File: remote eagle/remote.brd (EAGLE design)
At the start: 36.8 x 36.8 mm, 13 parts, among them U1 BLE112-A

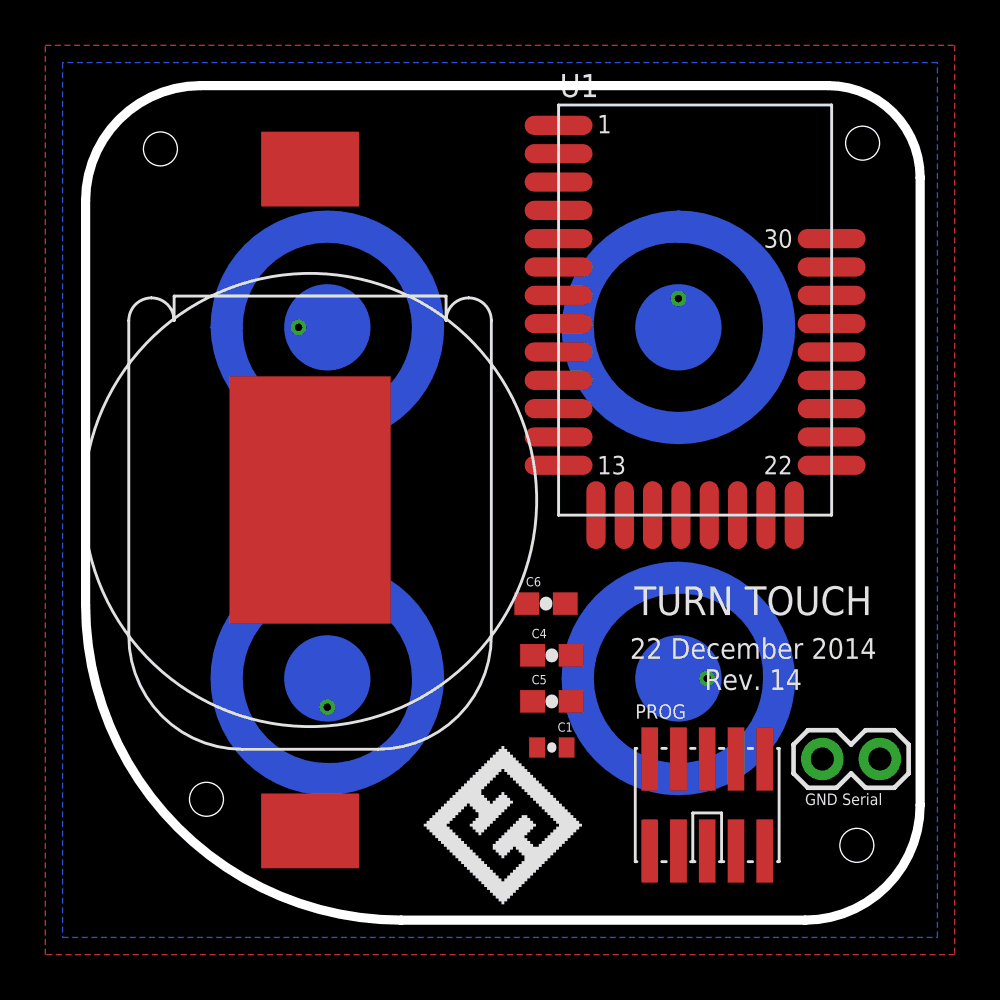
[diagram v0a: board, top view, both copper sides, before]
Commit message: Revision 14 of the board.
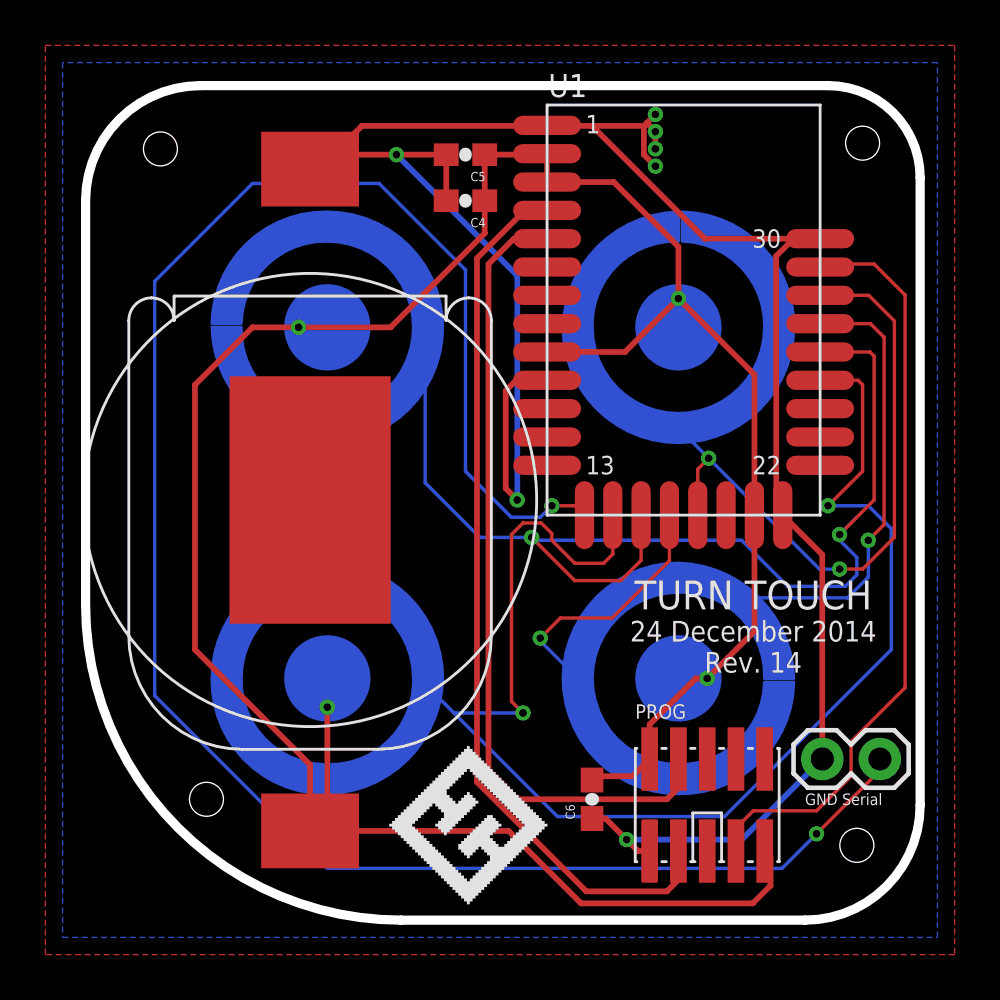
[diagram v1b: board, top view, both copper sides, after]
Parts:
- removed C1: .1uF, SparkFun-Passives:0402-CAP
- moved C5 24.4 mm to (16.8, 33.8), turned to 180 degrees
- moved C4 20.4 mm to (16.8, 31.8), turned to 180 degrees
- moved C6 8.87 mm to (22.4, 5.33), turned to 90 degrees
- moved LOGO 1.52 mm to (13.5, 0.76)
- moved U1 0.51 mm to (26.4, 26.9)
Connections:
- removed net 3.3V: C1.1, C4.1, C5.1, C6.2, PROG.2, PROG.9, U$1.P.C$1@1, U$1.P.C$1@2, U$2.P.C$1@1, U$2.P.C$1@2, U$3.P.C$1@1, U$3.P.C$1@2, U$4.P.C$1@1, U$4.P.C$1@2, U$6.P$1, U1.AVDD1, U1.AVDD2, U1.DVDD, U1.VDD_USB
- new net VCC: C4.1, C5.1, C6.2, PROG.2, PROG.9, U$1.P$1, U$1.P$2, U$2.P$1, U$2.P$2, U$3.P$1, U$3.P$2, U$4.P$1, U$4.P$2, U$6.P$1, U1.AVDD1, U1.AVDD2, U1.DVDD, U1.VDD_USB
- net BUTTON1: now also U$1.P$3; no longer U$1.P.O$1
- net BUTTON2: now also U$2.P$3; no longer U$2.P.O$1
- net BUTTON3: now also U$3.P$3; no longer U$3.P.O$1
- net BUTTON4: now also U$4.P$3; no longer U$4.P.O$1
- net GND: no longer C1.2
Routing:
- net VCC: track 0.00 -> 123.1 mm
- net GND: track 0.00 -> 103.3 mm, vias 0 -> 7
- net SERIAL: track 0.00 -> 88.2 mm, vias 0 -> 2
- net BUTTON4: track 0.00 -> 68.9 mm, vias 0 -> 2
- net BUTTON3: track 0.00 -> 50.2 mm, vias 0 -> 2
- net BUTTON2: track 0.00 -> 41.5 mm, vias 0 -> 2
- net P2_2: track 0.00 -> 40.3 mm
- net P2_1: track 0.00 -> 35.8 mm
- net RESET: track 0.00 -> 33.6 mm
- net BUTTON1: track 0.00 -> 28.7 mm, vias 0 -> 2
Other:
- board text added: "24 December 2014 Rev. 14"
- board text removed: "22 December 2014 Rev. 14"
